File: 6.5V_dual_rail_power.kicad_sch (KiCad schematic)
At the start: 26 parts, among them U2 TSR2-2465, U3 TSR2-2465

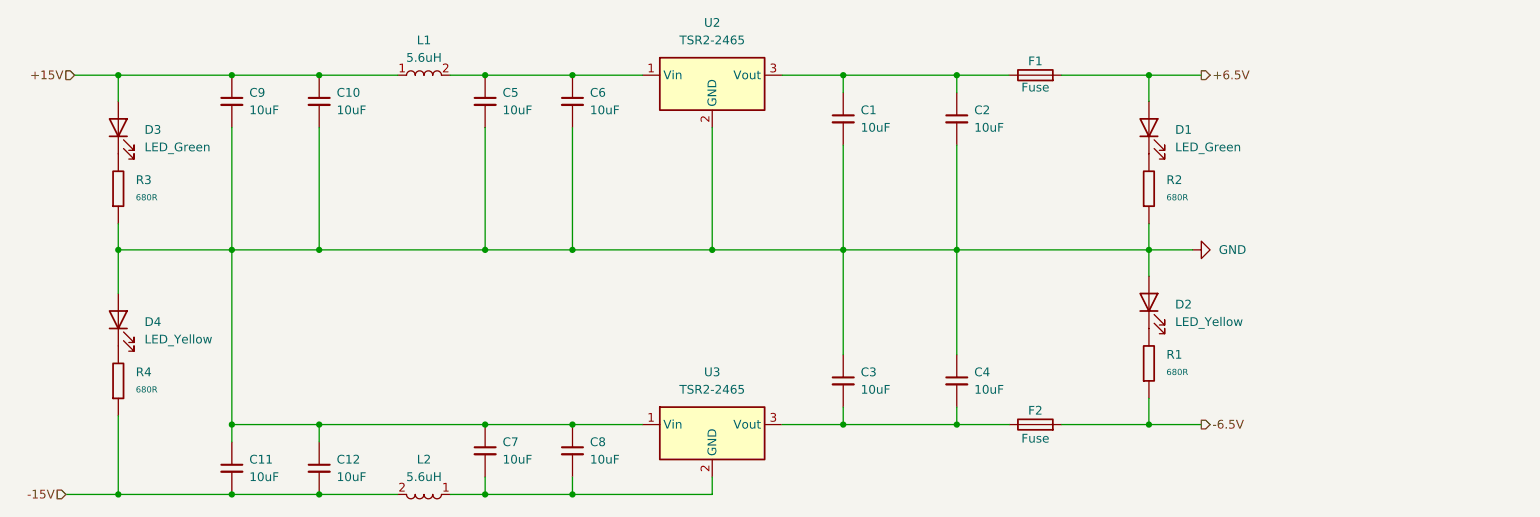
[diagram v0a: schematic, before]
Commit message: Added fab files.
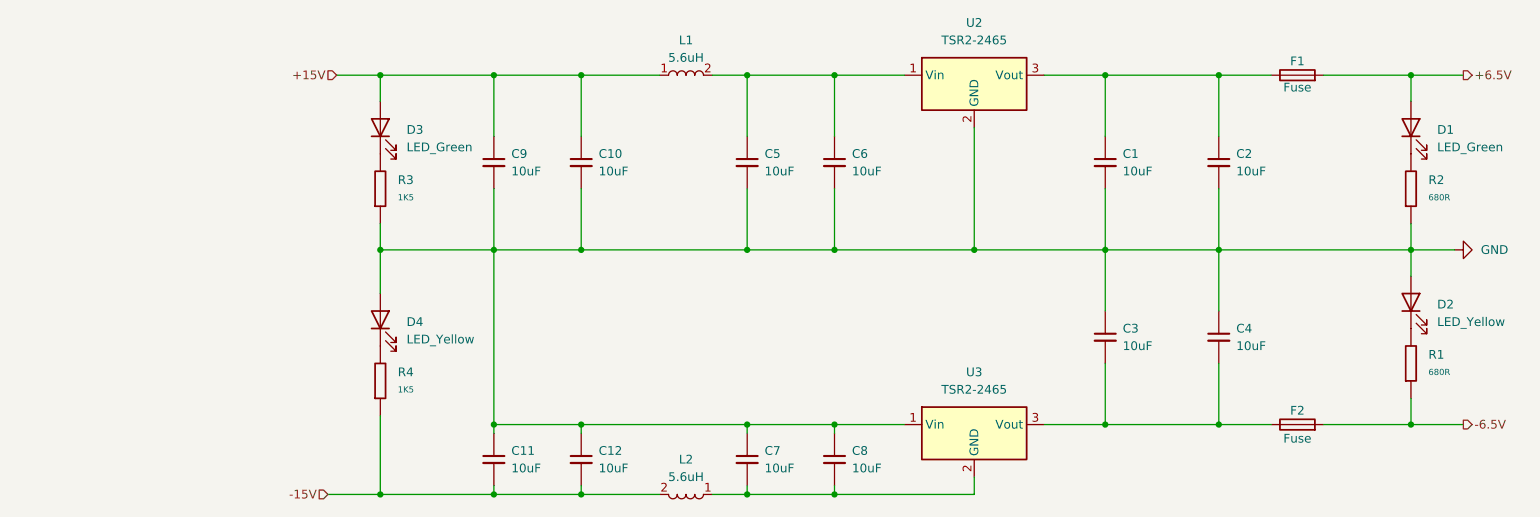
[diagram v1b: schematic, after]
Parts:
- D1, D2, D3, D4: Package/Footprint (none) -> LED_TH
- F1, F2: Package/Footprint (none) -> fuse_block
- L1, L2: Package/Footprint (none) -> tck_141; Type (none) -> SMD
- R3, R4: value 680R -> 1K5
- U2, U3: DigiKey Part Number (none) -> 1951-2427-ND; Manufacturer (none) -> Traco Power; Manufacturer Part Number (none) -> TSR 2-2465; Package/Footprint (none) -> 3-SIP Module; Type (none) -> thru-hole
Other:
- moved on the sheet: C1, C10, C11, C12, C2, C3, C4, C5, C6, C7, C8, C9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
